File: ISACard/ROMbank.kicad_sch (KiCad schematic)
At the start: 20 parts, among them U10 28C256, U6 74LS86, U7 74LS86, U8 74LS32, U9 74LS32

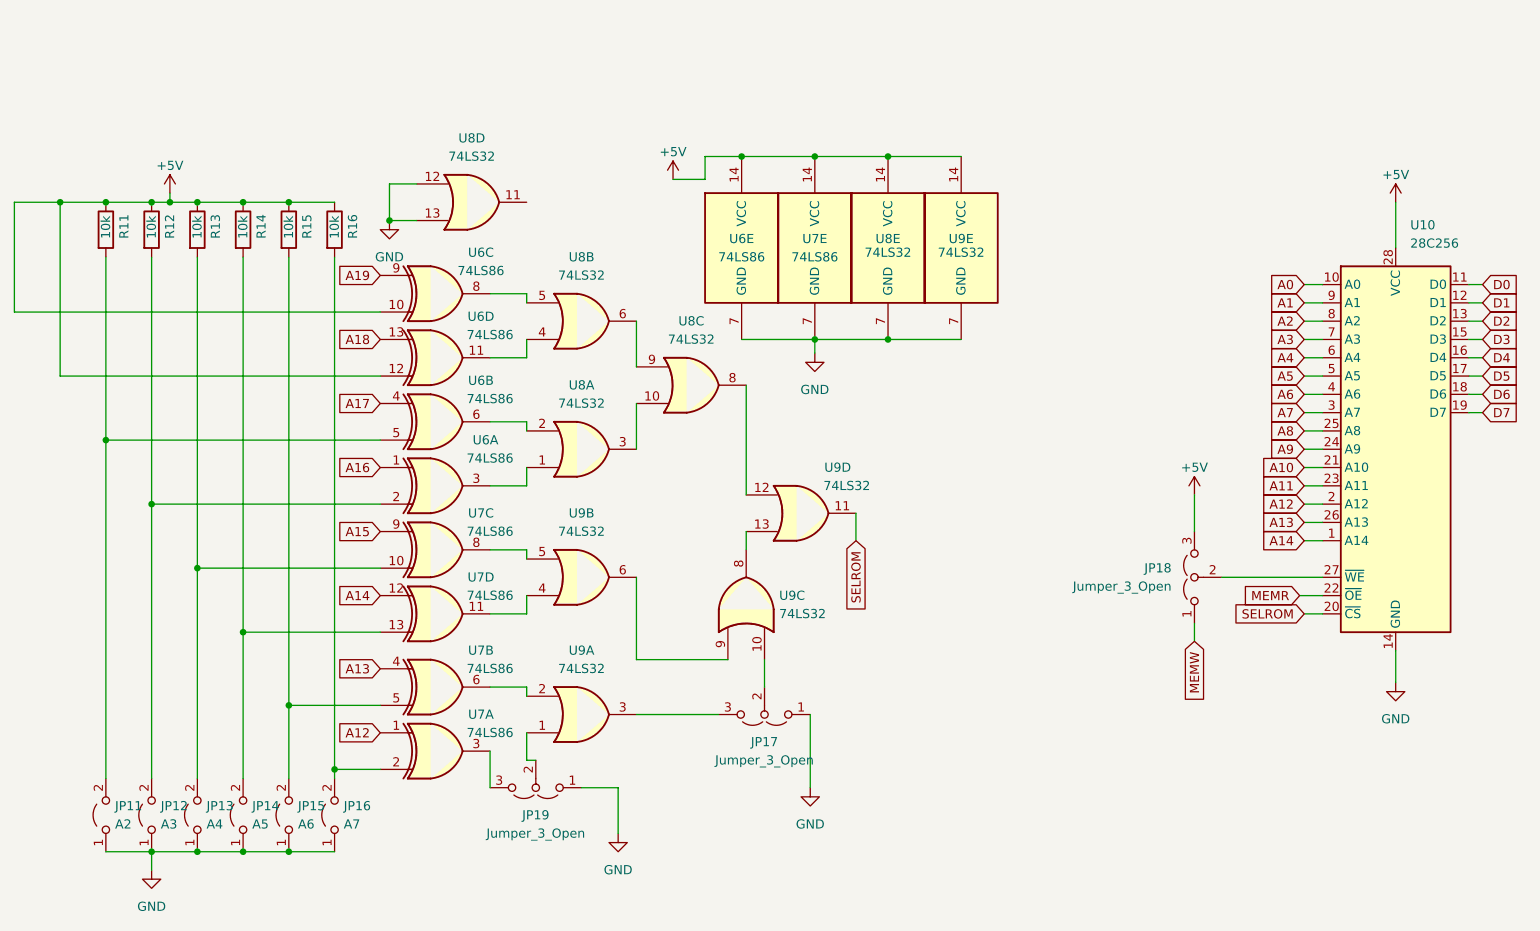
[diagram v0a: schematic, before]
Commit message: Fixed some problems with the card...
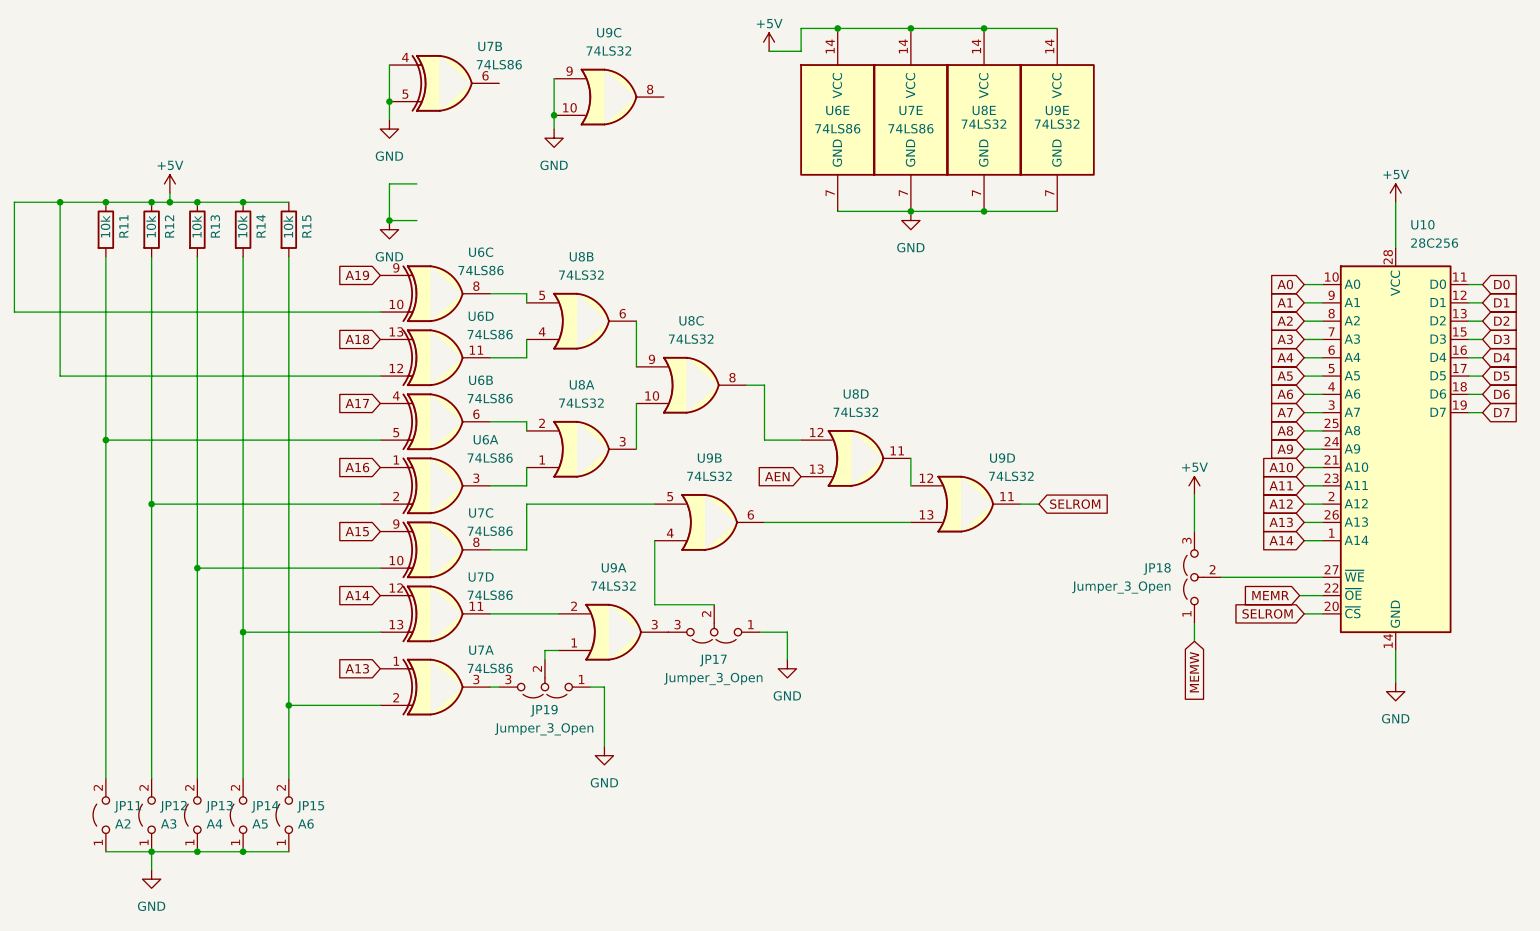
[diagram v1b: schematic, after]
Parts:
- removed JP16: A7, Connector_PinHeader_2.54mm:PinHeader_1x02_P2.54mm_Vertical, symbol Jumper:Jumper_2_Open
- removed R16: 10k, Resistor_THT:R_Axial_DIN0207_L6.3mm_D2.5mm_P7.62mm_Horizontal, symbol Device:R
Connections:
- net A12: no longer U7.1
- net A13: now also U7.1; no longer U7.4
- net GND: now also U7.4, U7.5, U9.10, U9.9; no longer U8.12, U8.13
- net at U9.2: now also U7.11; no longer U7.6
- net at U7.2: now also JP15.2 (B), R15.2
- net at JP17.2 (C): now also U9.4; no longer U9.10
- net at U9.8: no longer U9.13
- net at U9.6: now also U9.13; no longer U9.9
- net at U8.11: now also U9.12
- net at U8.8: now also U8.12; no longer U9.12
- new net AEN: U8.13
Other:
- moved on the sheet: JP17, JP19, U6E, U7A, U7B, U7E, U8D, U8E, U9A, U9B, U9C, U9D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
